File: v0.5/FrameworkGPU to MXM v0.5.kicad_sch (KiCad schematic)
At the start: 124 parts, among them J1 MXM3.0, U2 FXBeam, U54 BR24G32FVT-3GE2

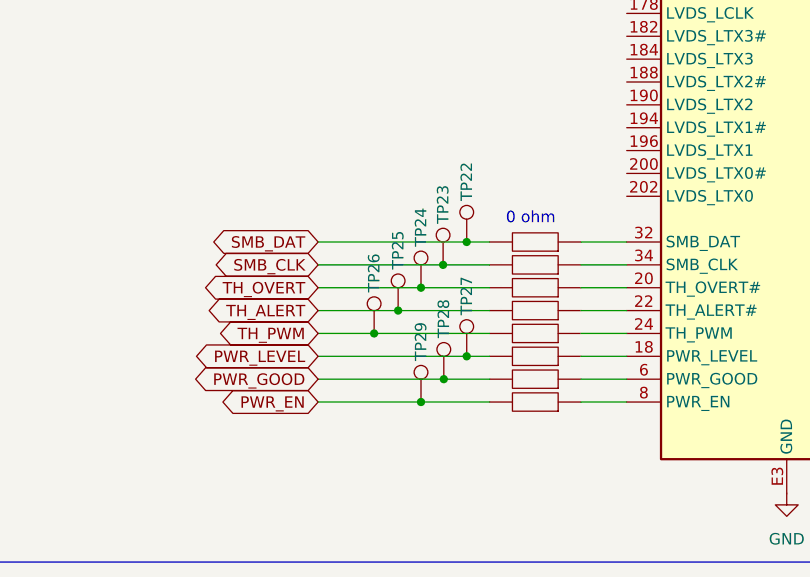
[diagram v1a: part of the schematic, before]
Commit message: committing final version sent off for manufacturing
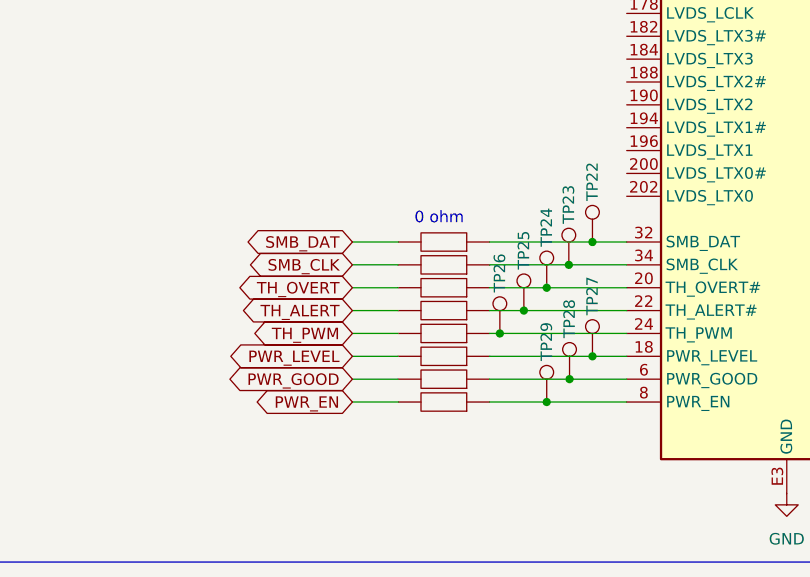
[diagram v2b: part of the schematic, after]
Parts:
- R17, R18, R19, R20, R21, R22, R23, R24, R25, R26, R27, R28, R29, R30, R31, R32: value 10K -> 0
- renumbered R1 to C1, R2 to C10, R5 to C11, R7 to C12, R9 to C13, R11 to C14, R13 to C15, R15 to C16, R4 to C2, R6 to C3, R8 to C4, R10 to C5, R12 to C6, R14 to C7, R16 to C8, R3 to C9
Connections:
- net PWR_EN: no longer TP29.1
- net PWR_GOOD: no longer TP28.1
- net PWR_LEVEL: no longer TP27.1
- net SMB_CLK: no longer TP23.1
- net SMB_DAT: no longer TP22.1
- net TH_ALERT: no longer TP25.1
- net TH_OVERT: no longer TP24.1
- net TH_PWM: no longer TP26.1
- net at J1.6 (PWR_GOOD), R63.1: now also TP28.1
- net at J1.32 (SMB_DAT), R55.1: now also TP22.1
- net at J1.18 (PWR_LEVEL), R62.1: now also TP27.1
- net at J1.22 (TH_ALERT#), R60.1: now also TP25.1
- net at J1.34 (SMB_CLK), R56.1: now also TP23.1
- net at J1.20 (TH_OVERT#), R59.1: now also TP24.1
- net at J1.24 (TH_PWM), R61.1: now also TP26.1
- net at J1.8 (PWR_EN), R64.1: now also TP29.1
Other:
- moved on the sheet: TP22, TP23, TP24, TP25, TP26, TP27, TP28, TP29
